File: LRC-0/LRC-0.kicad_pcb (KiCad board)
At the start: 4 copper layers, 100 x 100 mm, 57 parts, among them J1 USB_C_Receptacle_USB2.0_14P, J2 Battery, J3 Conn_01x10, J4 SMA, J5 u.FL, SW1 EN, SW2 BOOT, U1 AP7361C-33E, U2 TVS1400DRV, U3 BQ24075RGT, U4 ESP32-C6-MINI-1, U5 SX1262IMLTRT, U6 4259-63, U8 4259-63, Y1 TX32-33015S-32.000-X-R

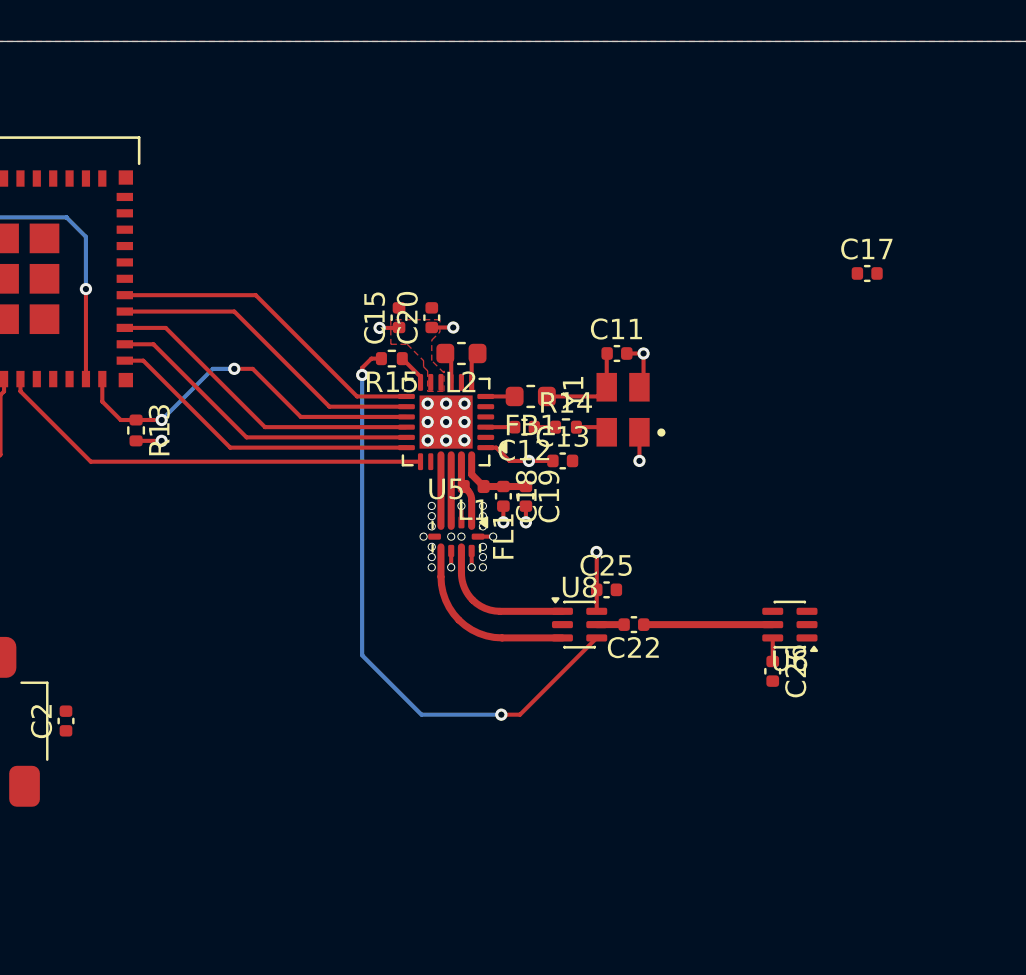
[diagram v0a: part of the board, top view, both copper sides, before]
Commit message: repositioning
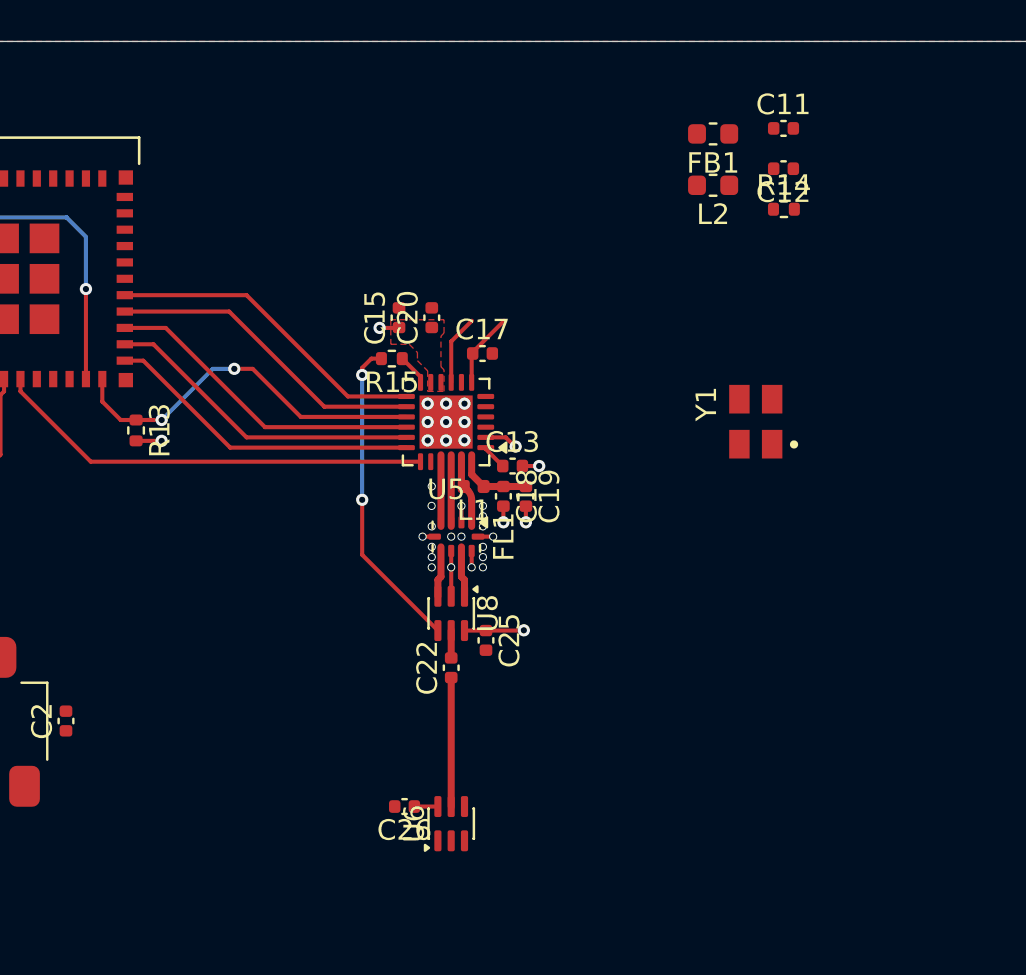
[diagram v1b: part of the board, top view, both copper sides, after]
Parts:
- moved C17 19.2 mm to (43.2, 15.2)
- moved U6 19.2 mm to (41.6, 38.2), turned to 90 degrees
- moved C26 19.2 mm to (39.4, 37.4), turned to 180 degrees
- moved C12 17.9 mm to (57.9, 6.22)
- moved FB1 15.6 mm to (54.5, 4.52)
- moved R14 15.1 mm to (57.9, 8.20)
- moved L2 14.8 mm to (54.5, 7.03)
- moved C11 13.7 mm to (57.9, 4.25)
- moved C22 9.18 mm to (41.6, 30.6), turned to 90 degrees
- moved Y1 6.51 mm to (56.5, 18.6)
- moved C25 6.39 mm to (43.4, 29.3), turned to -90 degrees
- moved U8 6.30 mm to (41.6, 28.0), turned to -90 degrees
- moved C13 2.46 mm to (44.6, 20.8)
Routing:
- net Net-(U8-CTRL): track 29.4 -> 15.5 mm
- net /RF1: track 9.08 -> 2.48 mm
- net /RF2: track 7.26 -> 2.48 mm
- net Net-(Y1-VDC): track 4.76 -> 0.00 mm
- net +3V3: track 14.5 -> 11.2 mm, vias 7 -> 5
- net Net-(U5-VREG): track 1.53 -> 3.67 mm
- net Net-(U5-DCC_SW): track 1.53 -> 3.43 mm
- net Net-(Y1-OUTPUT): track 1.58 -> 0.00 mm
- net /XTA: track 1.41 -> 0.00 mm
- net /DIO3: track 1.41 -> 0.00 mm
- net Net-(C12-Pad1): track 1.04 -> 0.00 mm

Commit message: first pass done
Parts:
- L2: footprint Inductor_SMD:L_0603_1608Metric -> Inductor_SMD:L_1008_2520Metric
- moved H1 139.6 mm to (119.2, 77.6)
- moved H2 139.6 mm to (119.2, 83.5)
- moved H3 139.6 mm to (119.2, 89.5)
- moved H4 139.6 mm to (119.2, 95.5)
- moved J3 139.6 mm to (113.9, 64.7)
- moved J4 61.0 mm to (34.9, 40.5), turned to -90 degrees
- moved J5 54.3 mm to (42.2, 35.4)
- moved C7 43.1 mm to (11.8, 35.3), turned to 90 degrees
- moved C6 42.3 mm to (10.8, 35.3), turned to 90 degrees
- moved R5 41.6 mm to (9.38, 34.4)
- moved C4 41.6 mm to (7.86, 33.1)
- moved D1 41.6 mm to (11.3, 38.4)
- moved D2 41.6 mm to (11.3, 40.6)
- moved R10 41.6 mm to (14.1, 38.4)
- moved R4 41.6 mm to (6.38, 31.6)
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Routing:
- net /ANT_CTRL: track 1.50 -> 32.9 mm, vias 1 -> 2
- net /BUSY: track 15.7 -> 8.02 mm
- net /SCK: track 15.5 -> 7.86 mm
- net /MISO: track 15.8 -> 8.10 mm
- net /DIO1: track 15.8 -> 8.15 mm
- net /MOSI: track 15.6 -> 7.98 mm
- net +3V3: track 11.2 -> 18.2 mm, vias 5 -> 7
- net Net-(Y1-VDC): track 0.00 -> 6.09 mm
- net GND: track 22.1 -> 27.4 mm, vias 51 -> 54
- net /ANT2: track 0.00 -> 5.12 mm
- net Net-(Y1-OUTPUT): track 0.00 -> 5.02 mm
- net /NRESET: track 18.3 -> 13.7 mm
- net /NSS: track 21.6 -> 16.9 mm
- net /ANT1: track 0.00 -> 4.52 mm
- net VCC: track 5.72 -> 1.93 mm, vias 0 -> 1
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- added copper zone on F.Cu, net /BAT+
- added copper zone on F.Cu, net VCC
- removed copper zone on F.Cu, net +3V3
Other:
- board size 100 x 100 mm -> 50 x 38.5 mm
